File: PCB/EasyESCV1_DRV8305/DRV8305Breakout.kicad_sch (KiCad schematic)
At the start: 39 parts, among them Q1 CSD16556Q5B, Q2 CSD16556Q5B, Q3 CSD16556Q5B, Q4 CSD16556Q5B, Q5 CSD16556Q5B, Q6 CSD16556Q5B, U1 DRV83053PHP, U3 TPD4E05U06DQAR

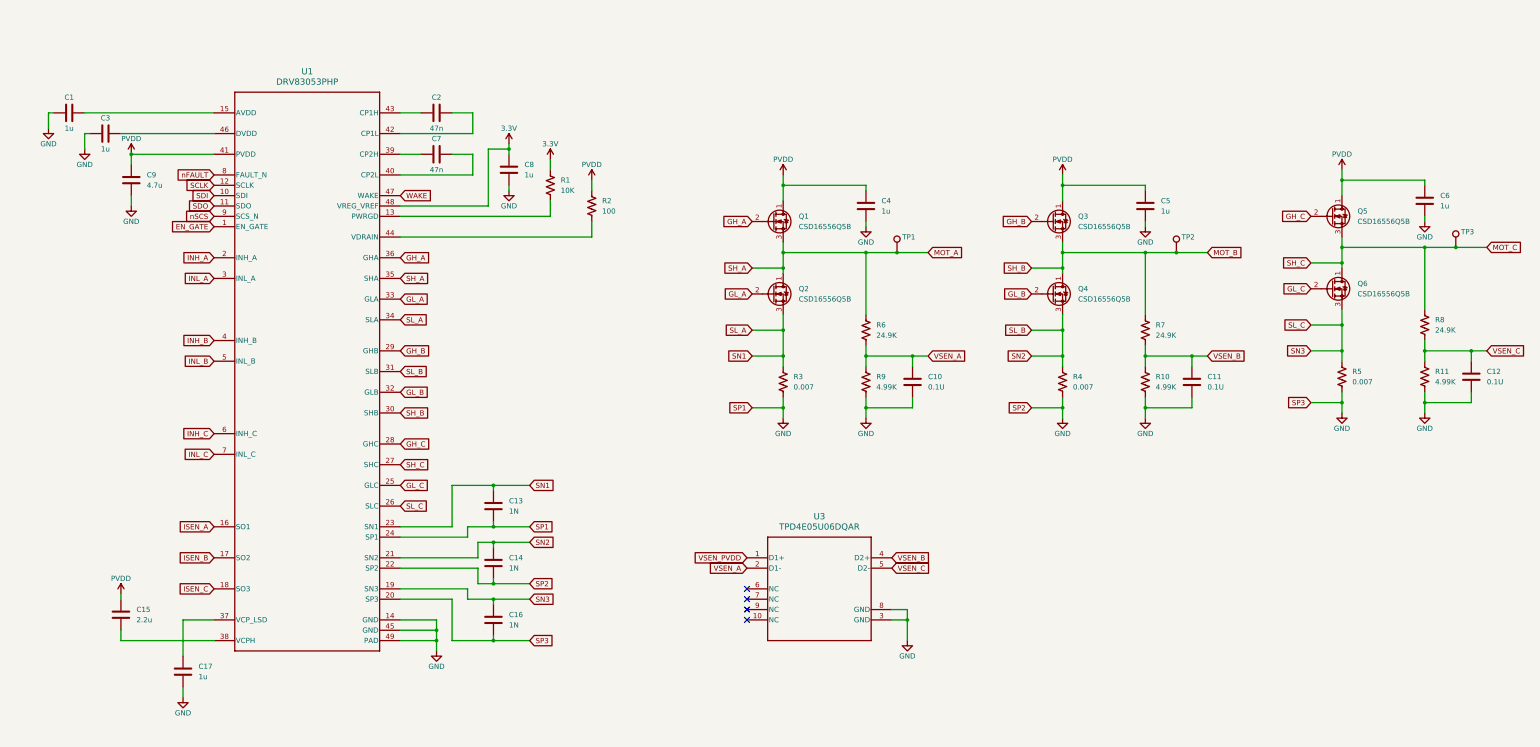
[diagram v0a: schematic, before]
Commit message: Finished REV1 Schematic Awaiting Review
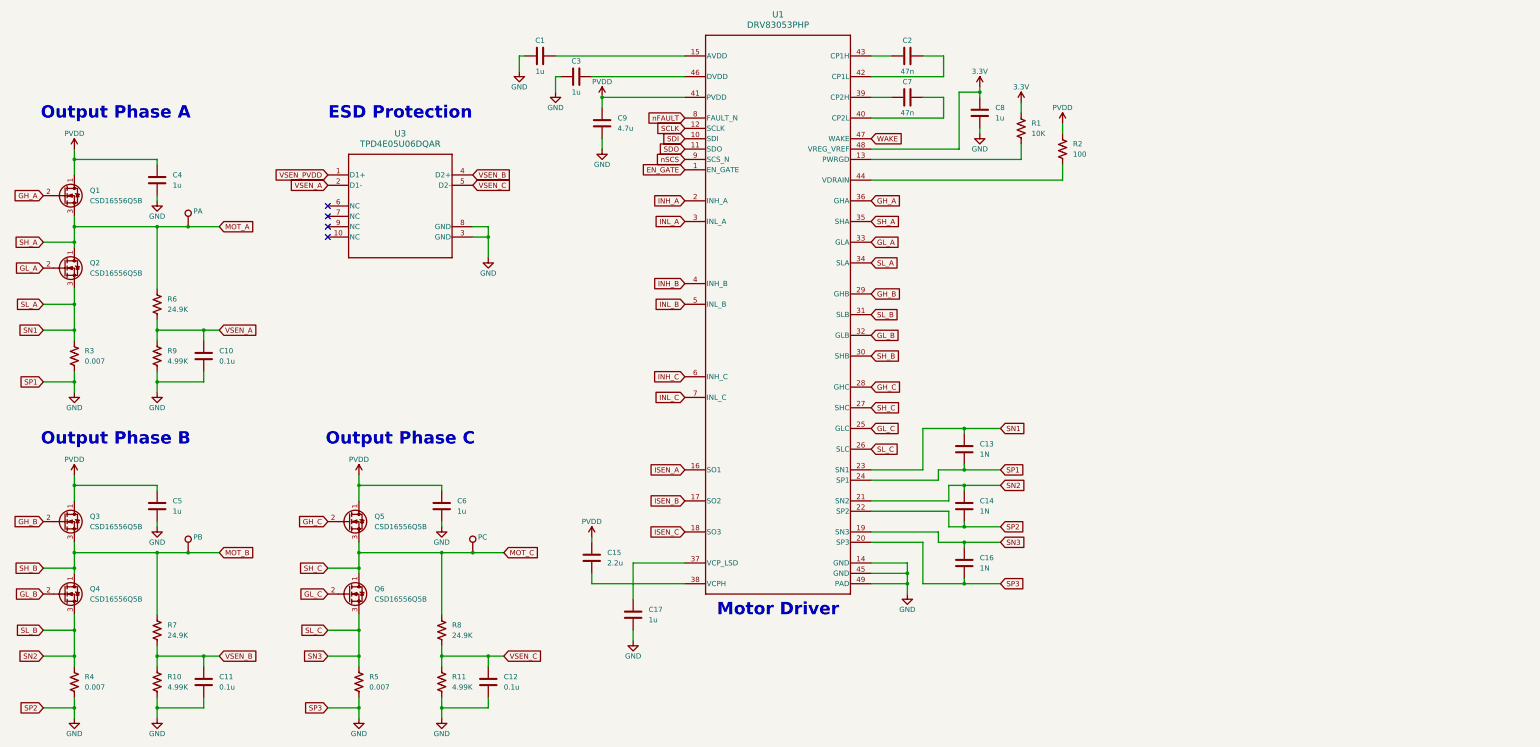
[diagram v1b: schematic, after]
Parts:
- C10, C11, C12: value 0.1U -> 0.1u
- renumbered TP1 to PA, TP2 to PB, TP3 to PC
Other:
- note added: "ESD Protection"
- note added: "Motor Driver"
- note added: "Output Phase A"
- note added: "Output Phase B"
- note added: "Output Phase C"
- company: (none) -> Buckley Boards 
- title: (none) -> Easy ESC
- moved on the sheet: C1, C10, C11, C12, C13, C14, C15, C16, C17, C2, C3, C4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
